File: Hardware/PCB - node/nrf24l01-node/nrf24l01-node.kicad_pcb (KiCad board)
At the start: 2 copper layers, 36.3 x 41.7 mm, 23 parts, among them IC1 ATSAMD21G18A-AU, IC2 TLP5010, U1 NRF24L01_Breakout, U2 BME280

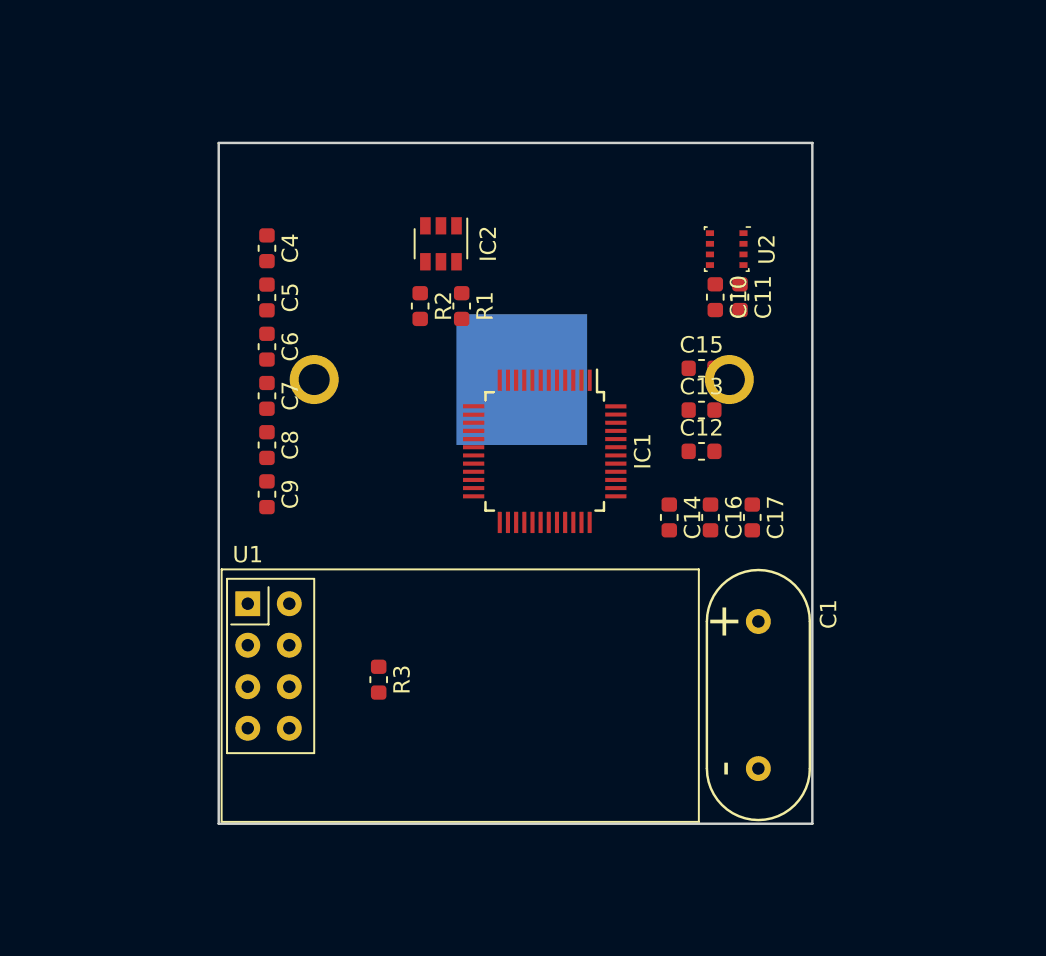
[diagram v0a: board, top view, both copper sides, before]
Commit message: Initial Hardware commit
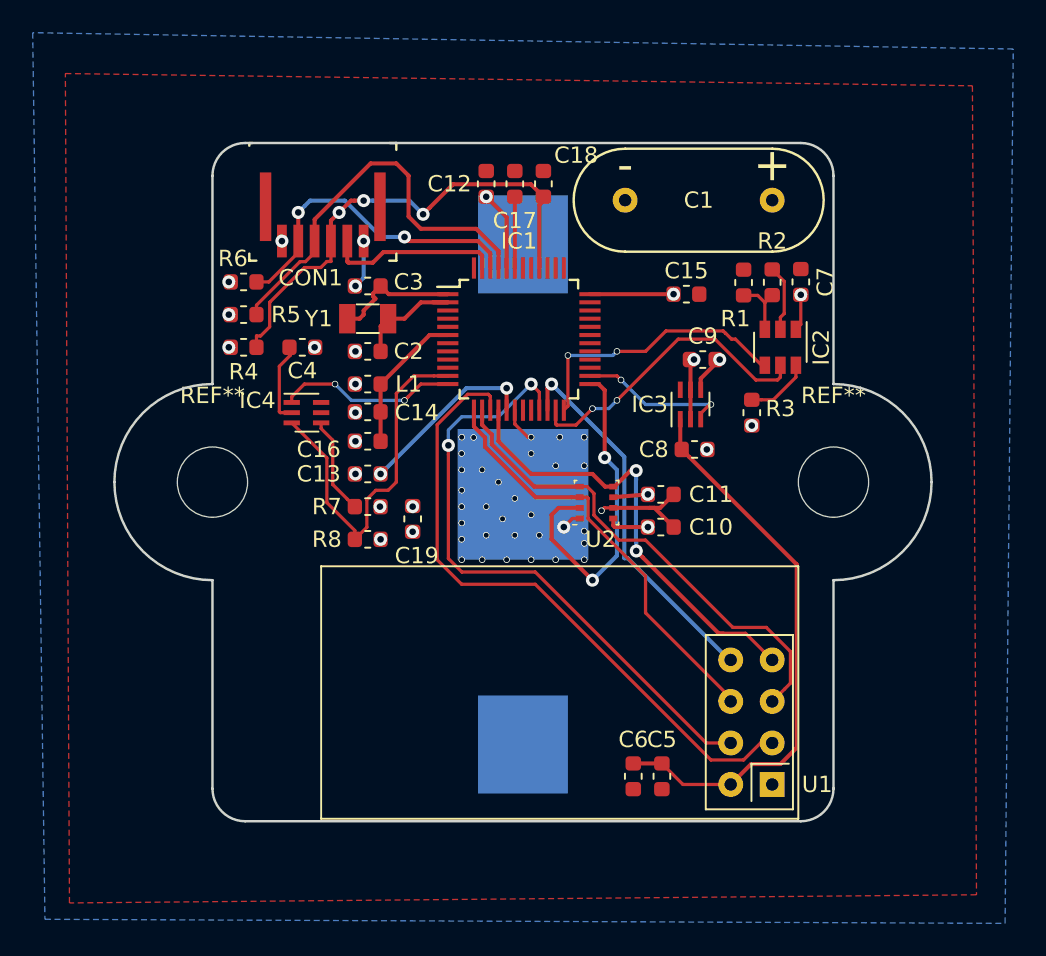
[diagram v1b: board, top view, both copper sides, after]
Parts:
- added C18: 100nF, Capacitor_SMD:C_0603_1608Metric, F.Cu at (76.0, 129.2)
- added C19: 100nF, Capacitor_SMD:C_0603_1608Metric, F.Cu at (68.0, 149.8)
- added C2: 15pF, Capacitor_SMD:C_0603_1608Metric, F.Cu at (65.2, 139.5)
- added C3: 15pF, Capacitor_SMD:C_0603_1608Metric, F.Cu at (65.2, 135.5)
- added CON1: FPC_6POS, FPC_conn:HFW6R_2STE1LF, F.Cu at (62.5, 132.2)
- added IC3: SIP32431, athir:SC-70-6, F.Cu at (85.0, 142.8)
- added IC4: SIP32431, athir:SC-70-6, F.Cu at (61.5, 143.2)
- added L1: SMD-FERRITE-CHIP-120-OHM-500MA_0603_, Capacitor_SMD:C_0603_1608Metric, F.Cu at (65.2, 141.5)
- added R4: 100k, Resistor_SMD:R_0603_1608Metric, F.Cu at (57.7, 139.2)
- added R5: 100k, Resistor_SMD:R_0603_1608Metric, F.Cu at (57.7, 137.2)
- added R6: 100k, Resistor_SMD:R_0603_1608Metric, F.Cu at (57.7, 135.2)
- added R7: 100k, Resistor_SMD:R_0603_1608Metric, F.Cu at (65.2, 149.0)
- added R8: 1M, Resistor_SMD:R_0603_1608Metric, F.Cu at (65.2, 151.0)
- added REF**: MountingHole_4.3mm_M4---PASTY, athir:MountingHole_4.3mm_M4---PASTY, F.Cu at (55.8, 147.5)
- added REF**: MountingHole_4.3mm_M4---PASTY, athir:MountingHole_4.3mm_M4---PASTY, F.Cu at (93.8, 147.5)
- added Y1: Crystal_Small, Crystal:Crystal_SMD_3215-2Pin_3.2x1.5mm, F.Cu at (65.2, 137.5)
- BT1: footprint Battery:BatteryHolder_Keystone_3009_1x2450 -> Battery:BatteryHolder_Keystone_3008_1x2450
- C4: value C_Small -> 100nF
- moved C5 38.0 mm to (83.2, 165.5)
- moved C6 34.5 mm to (81.5, 165.5)
- moved U1 33.9 mm to (90.0, 166.0), turned to 180 degrees
- moved C7 33.4 mm to (91.8, 135.2), turned to 90 degrees
- moved C1 30.5 mm to (85.5, 130.2), turned to 0 degrees
- moved R3 28.1 mm to (88.8, 143.2), turned to 90 degrees
- moved C9 27.9 mm to (85.8, 140.0), turned to 0 degrees
- moved C8 26.2 mm to (85.2, 145.5), turned to 0 degrees
- moved C17 25.1 mm to (74.2, 129.2), turned to 90 degrees
- moved IC2 21.7 mm to (90.5, 139.2)
- moved R2 21.6 mm to (90.0, 135.3), turned to 90 degrees
- moved C16 21.5 mm to (65.2, 145.0), turned to 180 degrees
- moved C12 21.0 mm to (72.5, 129.2), turned to 90 degrees
- moved C13 20.8 mm to (65.2, 147.0), turned to 180 degrees
- moved C14 19.5 mm to (65.2, 143.2), turned to 180 degrees
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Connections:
- C4 pad 1: GND -> VCC
- C8 pad 2: Net-(C8-Pad2) -> GND
- C9 pad 1: Net-(C8-Pad2) -> GND
- IC1 pad 11: Net-(IC1-Pad11) -> /VBAT_ADC_EN
- IC1 pad 12: Net-(IC1-Pad12) -> /VBAT_ADC
- IC1 pad 15: /NRF_SS -> /NRF_CE
- IC1 pad 21: /NRF_CE -> /NRF_CS
- IC1 pad 40: Net-(C4-Pad2) -> /MCU_RESET
- IC1 pad 47: Net-(IC1-Pad47) -> /UART_TX
- U1 pad 4: /NRF_SS -> /NRF_CS
- U2 pad 3: /BME280_SDA -> /BME280_SDI
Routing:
- net /NRF_CE: track 0.00 -> 39.2 mm
- net /NRF_CS: track 0.00 -> 37.8 mm, vias 0 -> 2
- net /NRF_VCC: track 0.00 -> 34.5 mm
- net VCC: track 0.00 -> 31.8 mm, vias 0 -> 17
- net /MCU_RESET: track 0.00 -> 30.3 mm, vias 0 -> 3
- net /BME280_SCK: track 0.00 -> 30.1 mm
- net /BME280_SDO: track 0.00 -> 27.9 mm, vias 0 -> 2
- net /BME280_SDI: track 0.00 -> 26.3 mm
- net /SWCLK: track 0.00 -> 24.9 mm
- net /NRF_IRQ: track 0.00 -> 23.4 mm, vias 0 -> 1
- net /VBAT_ADC_EN: track 0.00 -> 22.7 mm
- net GND: track 0.00 -> 20.9 mm, vias 0 -> 43
- net /BME280_SS: track 0.00 -> 20.5 mm, vias 0 -> 2
- net /SWDIO: track 0.00 -> 20.0 mm, vias 0 -> 2
- net /SIG_WAKE: track 0.00 -> 18.6 mm, vias 0 -> 2
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- added copper zone on F.Cu, net GND
- added copper zone on B.Cu, net VCC
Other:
- board size 36.3 x 41.7 mm -> 50 x 41.5 mm
- net class Default: clearance 0.2 -> 0.16; trace_width 0.25 -> 0.2
- rule trace_clearance: 0.2 -> 0.16
- board text removed: "1"
- board text removed: "4"
